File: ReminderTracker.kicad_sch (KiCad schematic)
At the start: 21 parts, among them J1 External RTC, SW1 SW_Push, SW2 SW_Push, SW3 SW_Push, SW4 SW_Push, SW5 SW_Push, SW6 SW_Push, U1 XIAO-ESP32-C3-DIP

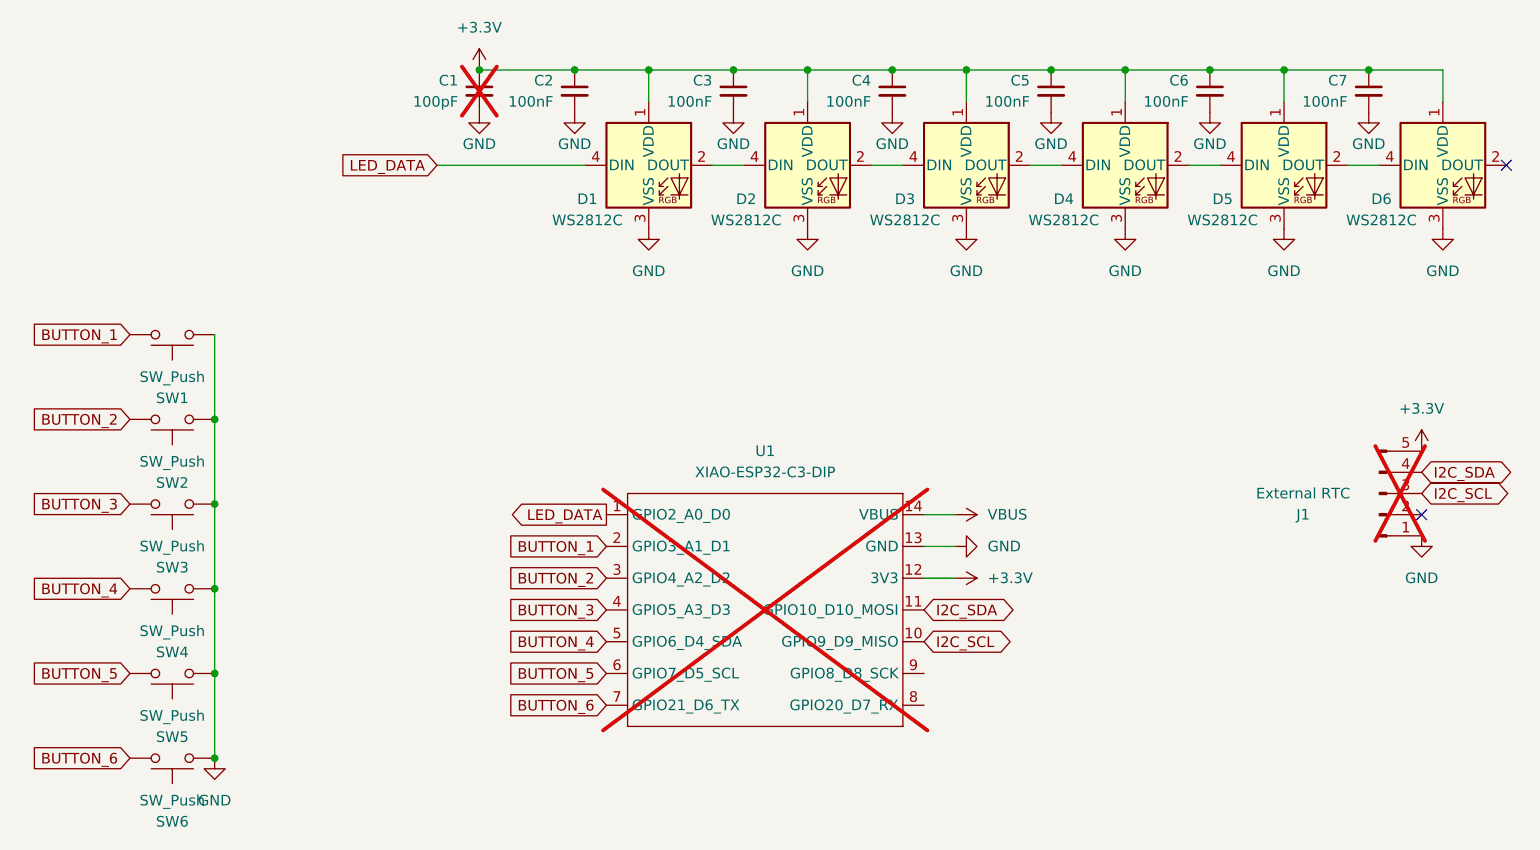
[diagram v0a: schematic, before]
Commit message: Revert "fix some things"
This reverts commit 1e6a08e8d2bd385bda99e6b5b2198f89c5206098.
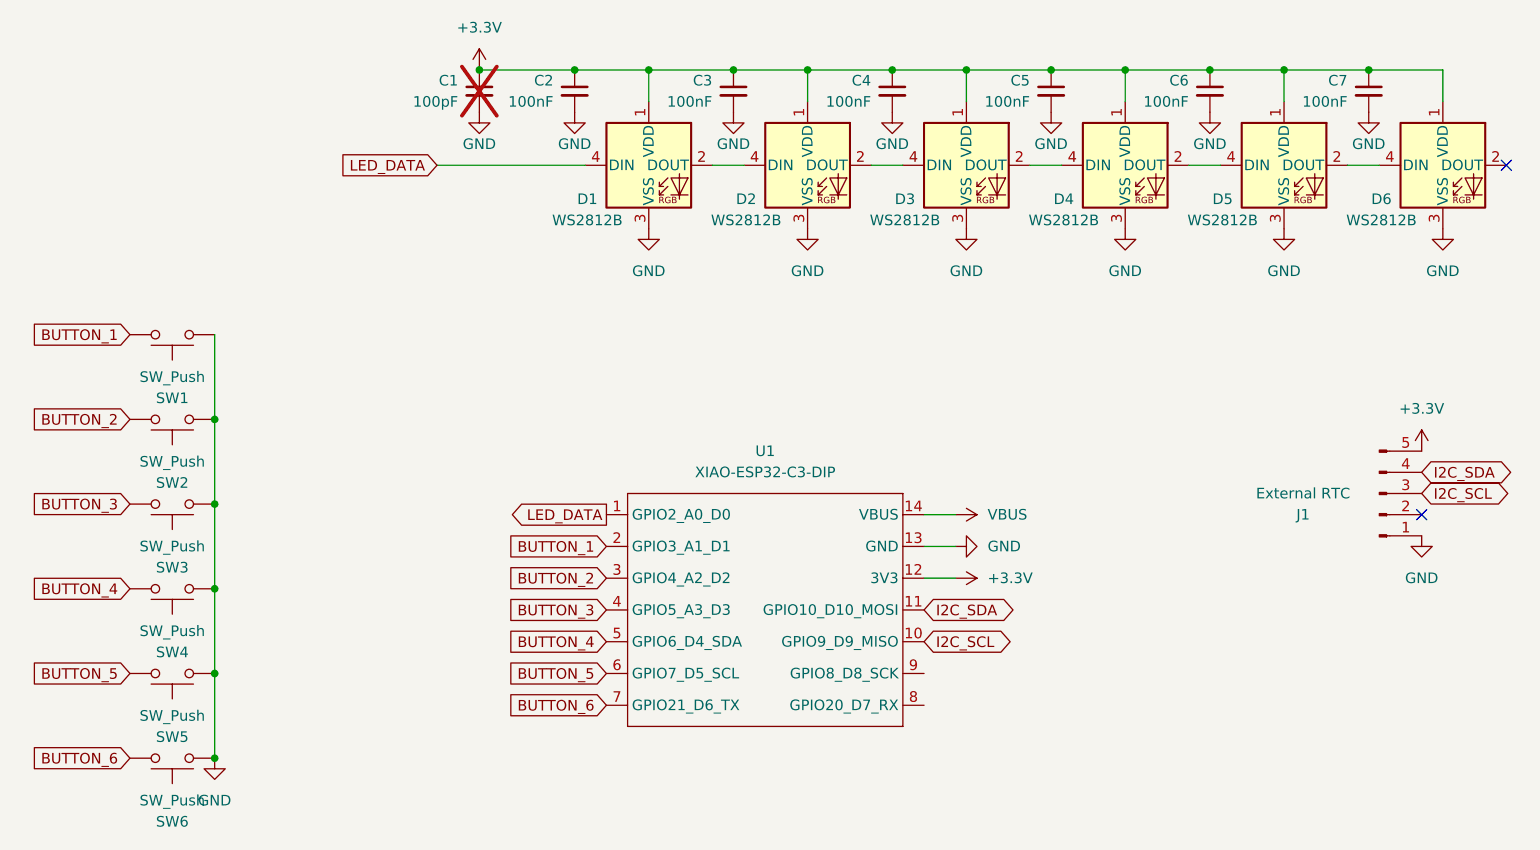
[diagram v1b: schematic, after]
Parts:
- C2, C3, C4, C5, C6, C7: LCSC Part # C24497 -> (none)
- D1, D2, D3, D4, D5, D6: value WS2812C -> WS2812B; LCSC Part # C42417624 -> (none)
- J1, U1: now fitted; now in the parts list
- SW1, SW2, SW3, SW4, SW5, SW6: LCSC Part # C13828 -> (none)
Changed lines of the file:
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@@
-			)
-		)
-		(property "LCSC Part #" "C24497"
-			(at 156.21 24.13 0)
-			(effects
-				(font
-					(size 1.27 1.27)
-				)
-				(hide yes)
 			)
 		)
@@
 			)
 		)
-		(property "Value" "WS2812C"
+		(property "Value" "WS2812B"
 			(at 195.834 39.624 0)
 			(effects
@@
 		)
 		(property "Description" "RGB LED with integrated controller"
-			(at 203.2 33.02 0)
-			(effects
-				(font
-					(size 1.27 1.27)
-				)
-				(hide yes)
-			)
-		)
-		(property "LCSC Part #" "C42417624"
 			(at 203.2 33.02 0)
 			(effects
@@
 			)
 		)
-		(property "LCSC Part #" "C13828"
-			(at 50.8 63.5 0)
-			(effects
-				(font
-					(size 1.27 1.27)
-				)
-				(hide yes)
-			)
-		)
 		(pin "1"
 		)
@@
 			)
 		)
-		(property "Value" "WS2812C"
+		(property "Value" "WS2812B"
 			(at 119.634 39.624 0)
 			(effects
@@
 		)
 		(property "Description" "RGB LED with integrated controller"
-			(at 127 33.02 0)
-			(effects
-				(font
-					(size 1.27 1.27)
-				)
-				(hide yes)
-			)
-		)
-		(property "LCSC Part #" "C42417624"
 			(at 127 33.02 0)
 			(effects
@@
 		(unit 1)
 		(exclude_from_sim no)
-		(in_bom no)
-		(on_board yes)
-		(dnp yes)
+		(in_bom yes)
+		(on_board yes)
+		(dnp no)
 		(property "Reference" "J1"
 			(at 186.436 74.93 0)
@@
 			)
 		)
-		(property "LCSC Part #" "C24497"
-			(at 99.06 24.13 0)
-			(effects
-				(font
-					(size 1.27 1.27)
-				)
-				(hide yes)
-			)
-		)
 		(pin "1"
 		)
@@
 		)
 		(property "Description" "Unpolarized capacitor, small symbol"
-			(at 137.16 24.13 0)
-			(effects
-				(font
-					(size 1.27 1.27)
-				)
-				(hide yes)
-			)
-		)
-		(property "LCSC Part #" "C24497"
 			(at 137.16 24.13 0)
 			(effects
@@
 			)
 		)
-		(property "LCSC Part #" "C13828"
-			(at 50.8 53.34 0)
-			(effects
-				(font
-					(size 1.27 1.27)
-				)
-				(hide yes)
-			)
-		)
 		(pin "1"
 		)
@@
 		(unit 1)
 		(exclude_from_sim no)
-		(in_bom no)
-		(on_board yes)
-		(dnp yes)
+		(in_bom yes)
+		(on_board yes)
+		(dnp no)
 		(fields_autoplaced yes)
 		(property "Reference" "U1"
@@
 			)
 		)
-		(property "LCSC Part #" "C13828"
-			(at 50.8 73.66 0)
-			(effects
-				(font
-					(size 1.27 1.27)
-				)
-				(hide yes)
-			)
-		)
 		(pin "1"
 		)
@@
 			)
 		)
-		(property "LCSC Part #" "C13828"
-			(at 50.8 104.14 0)
-			(effects
-				(font
-					(size 1.27 1.27)
-				)
-				(hide yes)
-			)
-		)
 		(pin "1"
 		)
@@
 			)
 		)
-		(property "LCSC Part #" "C24497"
-			(at 118.11 24.13 0)
-			(effects
-				(font
-					(size 1.27 1.27)
-				)
-				(hide yes)
-			)
-		)
 		(pin "1"
 		)
@@
 			)
 		)
-		(property "Value" "WS2812C"
+		(property "Value" "WS2812B"
 			(at 176.784 39.624 0)
 			(effects
@@
 		)
 		(property "Description" "RGB LED with integrated controller"
-			(at 184.15 33.02 0)
-			(effects
-				(font
-					(size 1.27 1.27)
-				)
-				(hide yes)
-			)
-		)
-		(property "LCSC Part #" "C42417624"
 			(at 184.15 33.02 0)
 			(effects
@@
 			)
 		)
-		(property "Value" "WS2812C"
+		(property "Value" "WS2812B"
 			(at 138.684 39.624 0)
 			(effects
@@
 		)
 		(property "Description" "RGB LED with integrated controller"
-			(at 146.05 33.02 0)
-			(effects
-				(font
-					(size 1.27 1.27)
-				)
-				(hide yes)
-			)
-		)
-		(property "LCSC Part #" "C42417624"
 			(at 146.05 33.02 0)
 			(effects
@@
 			)
 		)
-		(property "LCSC Part #" "C13828"
-			(at 50.8 93.98 0)
-			(effects
-				(font
-					(size 1.27 1.27)
-				)
-				(hide yes)
-			)
-		)
 		(pin "1"
 		)
@@
 			)
 		)
-		(property "Value" "WS2812C"
+		(property "Value" "WS2812B"
 			(at 100.584 39.624 0)
 			(effects
@@
 		)
 		(property "Description" "RGB LED with integrated controller"
-			(at 107.95 33.02 0)
-			(effects
-				(font
-					(size 1.27 1.27)
-				)
-				(hide yes)
-			)
-		)
-		(property "LCSC Part #" "C42417624"
 			(at 107.95 33.02 0)
 			(effects
@@
 			)
 		)
-		(property "LCSC Part #" "C24497"
-			(at 175.26 24.13 0)
-			(effects
-				(font
-					(size 1.27 1.27)
-				)
-				(hide yes)
-			)
-		)
 		(pin "1"
 		)
@@
 			)
 		)
-		(property "LCSC Part #" "C24497"
-			(at 194.31 24.13 0)
-			(effects
-				(font
-					(size 1.27 1.27)
-				)
-				(hide yes)
-			)
-		)
 		(pin "1"
 		)
@@
 			)
 		)
-		(property "LCSC Part #" "C13828"
-			(at 50.8 83.82 0)
-			(effects
-				(font
-					(size 1.27 1.27)
-				)
-				(hide yes)
-			)
-		)
 		(pin "1"
 		)
@@
 			)
 		)
-		(property "Value" "WS2812C"
+		(property "Value" "WS2812B"
 			(at 157.734 39.624 0)
 			(effects
@@
 			(at 165.1 33.02 0)
 			(effects
-				(font
-					(size 1.27 1.27)
-				)
-				(hide yes)
-			)
-		)
-		(property "LCSC Part #" "C42417624"
-			(at 165.1 33.02 0)
-			(effects

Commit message: fix some things
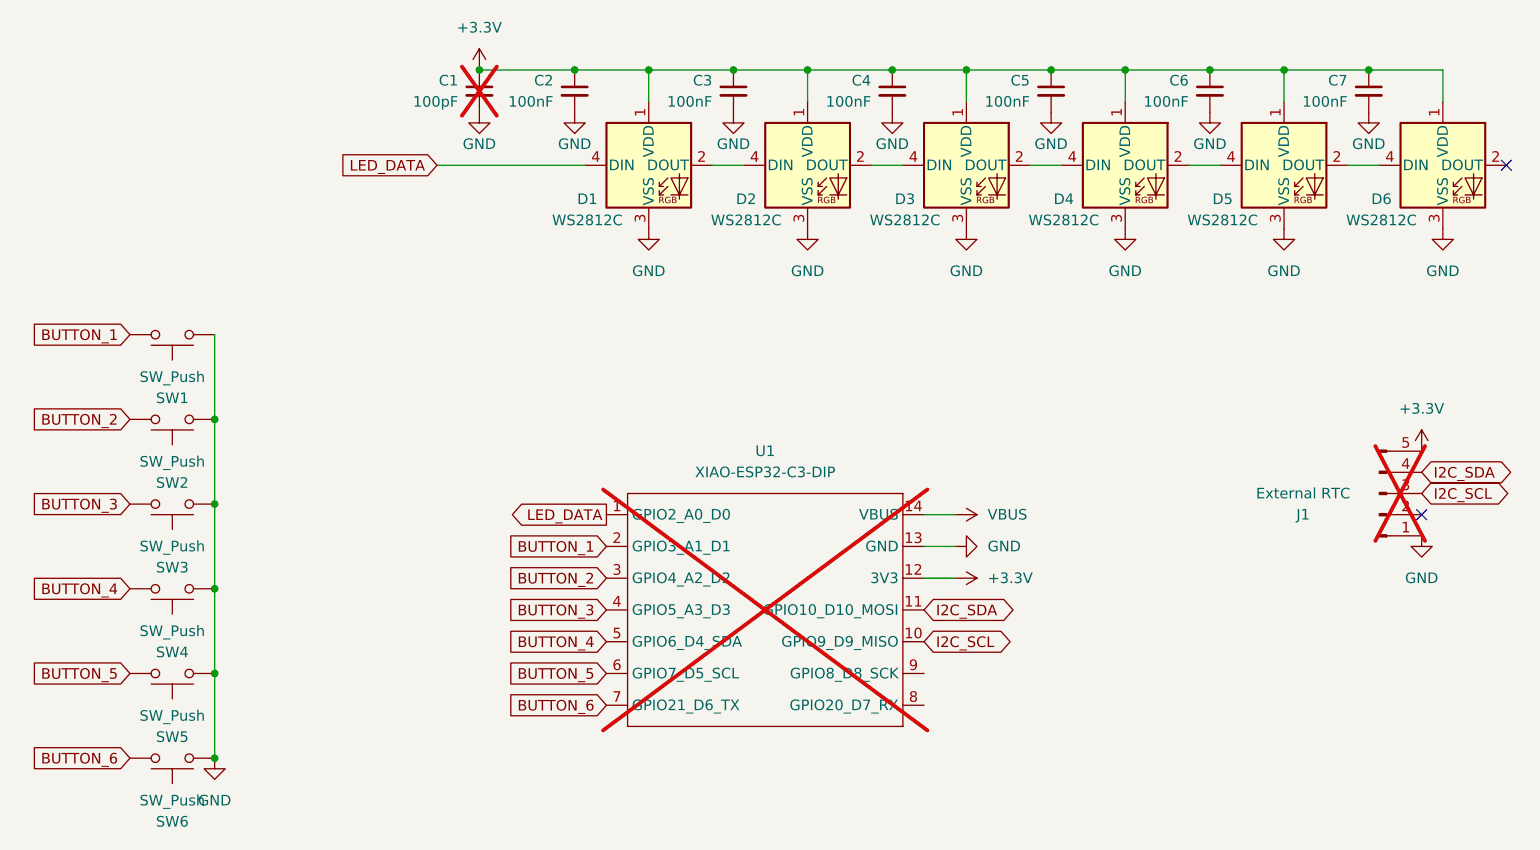
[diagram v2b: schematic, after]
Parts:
- C2, C3, C4, C5, C6, C7: LCSC Part # (none) -> C24497
- D1, D2, D3, D4, D5, D6: value WS2812B -> WS2812C; LCSC Part # (none) -> C42417624
- J1, U1: now not fitted; now left out of the parts list
- SW1, SW2, SW3, SW4, SW5, SW6: LCSC Part # (none) -> C13828
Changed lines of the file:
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@@
+			)
+		)
+		(property "LCSC Part #" "C24497"
+			(at 156.21 24.13 0)
+			(effects
+				(font
+					(size 1.27 1.27)
+				)
+				(hide yes)
 			)
 		)
@@
 			)
 		)
-		(property "Value" "WS2812B"
+		(property "Value" "WS2812C"
 			(at 195.834 39.624 0)
 			(effects
@@
 		)
 		(property "Description" "RGB LED with integrated controller"
+			(at 203.2 33.02 0)
+			(effects
+				(font
+					(size 1.27 1.27)
+				)
+				(hide yes)
+			)
+		)
+		(property "LCSC Part #" "C42417624"
 			(at 203.2 33.02 0)
 			(effects
@@
 			)
 		)
+		(property "LCSC Part #" "C13828"
+			(at 50.8 63.5 0)
+			(effects
+				(font
+					(size 1.27 1.27)
+				)
+				(hide yes)
+			)
+		)
 		(pin "1"
 		)
@@
 			)
 		)
-		(property "Value" "WS2812B"
+		(property "Value" "WS2812C"
 			(at 119.634 39.624 0)
 			(effects
@@
 		)
 		(property "Description" "RGB LED with integrated controller"
+			(at 127 33.02 0)
+			(effects
+				(font
+					(size 1.27 1.27)
+				)
+				(hide yes)
+			)
+		)
+		(property "LCSC Part #" "C42417624"
 			(at 127 33.02 0)
 			(effects
@@
 		(unit 1)
 		(exclude_from_sim no)
-		(in_bom yes)
-		(on_board yes)
-		(dnp no)
+		(in_bom no)
+		(on_board yes)
+		(dnp yes)
 		(property "Reference" "J1"
 			(at 186.436 74.93 0)
@@
 			)
 		)
+		(property "LCSC Part #" "C24497"
+			(at 99.06 24.13 0)
+			(effects
+				(font
+					(size 1.27 1.27)
+				)
+				(hide yes)
+			)
+		)
 		(pin "1"
 		)
@@
 		)
 		(property "Description" "Unpolarized capacitor, small symbol"
+			(at 137.16 24.13 0)
+			(effects
+				(font
+					(size 1.27 1.27)
+				)
+				(hide yes)
+			)
+		)
+		(property "LCSC Part #" "C24497"
 			(at 137.16 24.13 0)
 			(effects
@@
 			)
 		)
+		(property "LCSC Part #" "C13828"
+			(at 50.8 53.34 0)
+			(effects
+				(font
+					(size 1.27 1.27)
+				)
+				(hide yes)
+			)
+		)
 		(pin "1"
 		)
@@
 		(unit 1)
 		(exclude_from_sim no)
-		(in_bom yes)
-		(on_board yes)
-		(dnp no)
+		(in_bom no)
+		(on_board yes)
+		(dnp yes)
 		(fields_autoplaced yes)
 		(property "Reference" "U1"
@@
 			)
 		)
+		(property "LCSC Part #" "C13828"
+			(at 50.8 73.66 0)
+			(effects
+				(font
+					(size 1.27 1.27)
+				)
+				(hide yes)
+			)
+		)
 		(pin "1"
 		)
@@
 			)
 		)
+		(property "LCSC Part #" "C13828"
+			(at 50.8 104.14 0)
+			(effects
+				(font
+					(size 1.27 1.27)
+				)
+				(hide yes)
+			)
+		)
 		(pin "1"
 		)
@@
 			)
 		)
+		(property "LCSC Part #" "C24497"
+			(at 118.11 24.13 0)
+			(effects
+				(font
+					(size 1.27 1.27)
+				)
+				(hide yes)
+			)
+		)
 		(pin "1"
 		)
@@
 			)
 		)
-		(property "Value" "WS2812B"
+		(property "Value" "WS2812C"
 			(at 176.784 39.624 0)
 			(effects
@@
 		)
 		(property "Description" "RGB LED with integrated controller"
+			(at 184.15 33.02 0)
+			(effects
+				(font
+					(size 1.27 1.27)
+				)
+				(hide yes)
+			)
+		)
+		(property "LCSC Part #" "C42417624"
 			(at 184.15 33.02 0)
 			(effects
@@
 			)
 		)
-		(property "Value" "WS2812B"
+		(property "Value" "WS2812C"
 			(at 138.684 39.624 0)
 			(effects
@@
 		)
 		(property "Description" "RGB LED with integrated controller"
+			(at 146.05 33.02 0)
+			(effects
+				(font
+					(size 1.27 1.27)
+				)
+				(hide yes)
+			)
+		)
+		(property "LCSC Part #" "C42417624"
 			(at 146.05 33.02 0)
 			(effects
@@
 			)
 		)
+		(property "LCSC Part #" "C13828"
+			(at 50.8 93.98 0)
+			(effects
+				(font
+					(size 1.27 1.27)
+				)
+				(hide yes)
+			)
+		)
 		(pin "1"
 		)
@@
 			)
 		)
-		(property "Value" "WS2812B"
+		(property "Value" "WS2812C"
 			(at 100.584 39.624 0)
 			(effects
@@
 		)
 		(property "Description" "RGB LED with integrated controller"
+			(at 107.95 33.02 0)
+			(effects
+				(font
+					(size 1.27 1.27)
+				)
+				(hide yes)
+			)
+		)
+		(property "LCSC Part #" "C42417624"
 			(at 107.95 33.02 0)
 			(effects
@@
 			)
 		)
+		(property "LCSC Part #" "C24497"
+			(at 175.26 24.13 0)
+			(effects
+				(font
+					(size 1.27 1.27)
+				)
+				(hide yes)
+			)
+		)
 		(pin "1"
 		)
@@
 			)
 		)
+		(property "LCSC Part #" "C24497"
+			(at 194.31 24.13 0)
+			(effects
+				(font
+					(size 1.27 1.27)
+				)
+				(hide yes)
+			)
+		)
 		(pin "1"
 		)
@@
 			)
 		)
+		(property "LCSC Part #" "C13828"
+			(at 50.8 83.82 0)
+			(effects
+				(font
+					(size 1.27 1.27)
+				)
+				(hide yes)
+			)
+		)
 		(pin "1"
 		)
@@
 			)
 		)
-		(property "Value" "WS2812B"
+		(property "Value" "WS2812C"
 			(at 157.734 39.624 0)
 			(effects
@@
 			(at 165.1 33.02 0)
 			(effects
+				(font
+					(size 1.27 1.27)
+				)
+				(hide yes)
+			)
+		)
+		(property "LCSC Part #" "C42417624"
+			(at 165.1 33.02 0)
+			(effects
